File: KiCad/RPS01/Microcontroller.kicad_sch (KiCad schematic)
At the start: 24 parts, among them J1 ISCP, J2 Serial, J22 RGB LED, J3 i2c, J4 Aref, J5 XT30, J6 Temperture, J7 GPIO, SW1 MCU_Button, U1 ATmega328P-A, U2 AMS1117, U3 ADR02AUJZ-REEL7, Y1 16Mhz Crystal

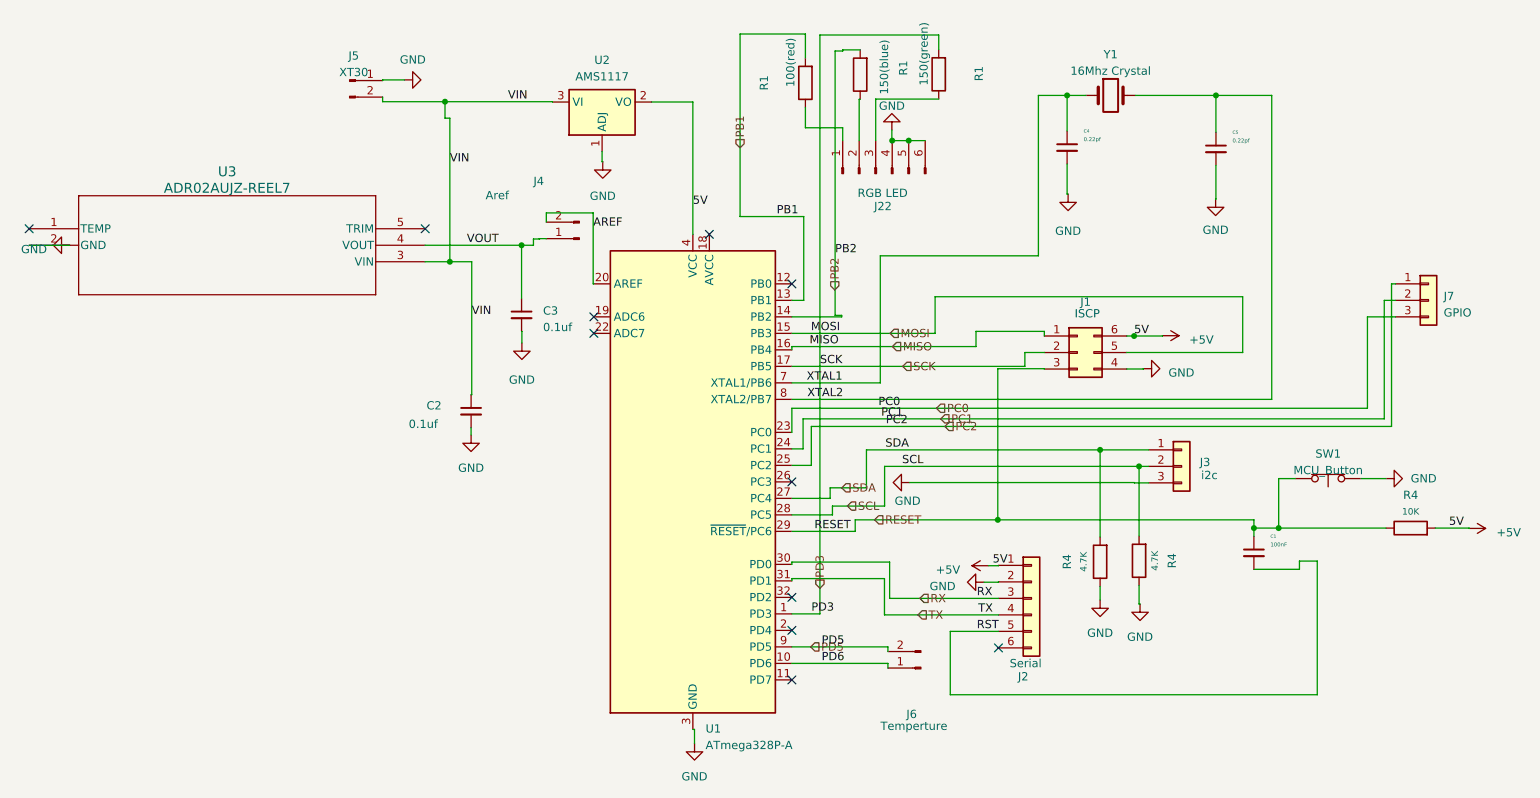
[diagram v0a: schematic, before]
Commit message: Large Schematic Update
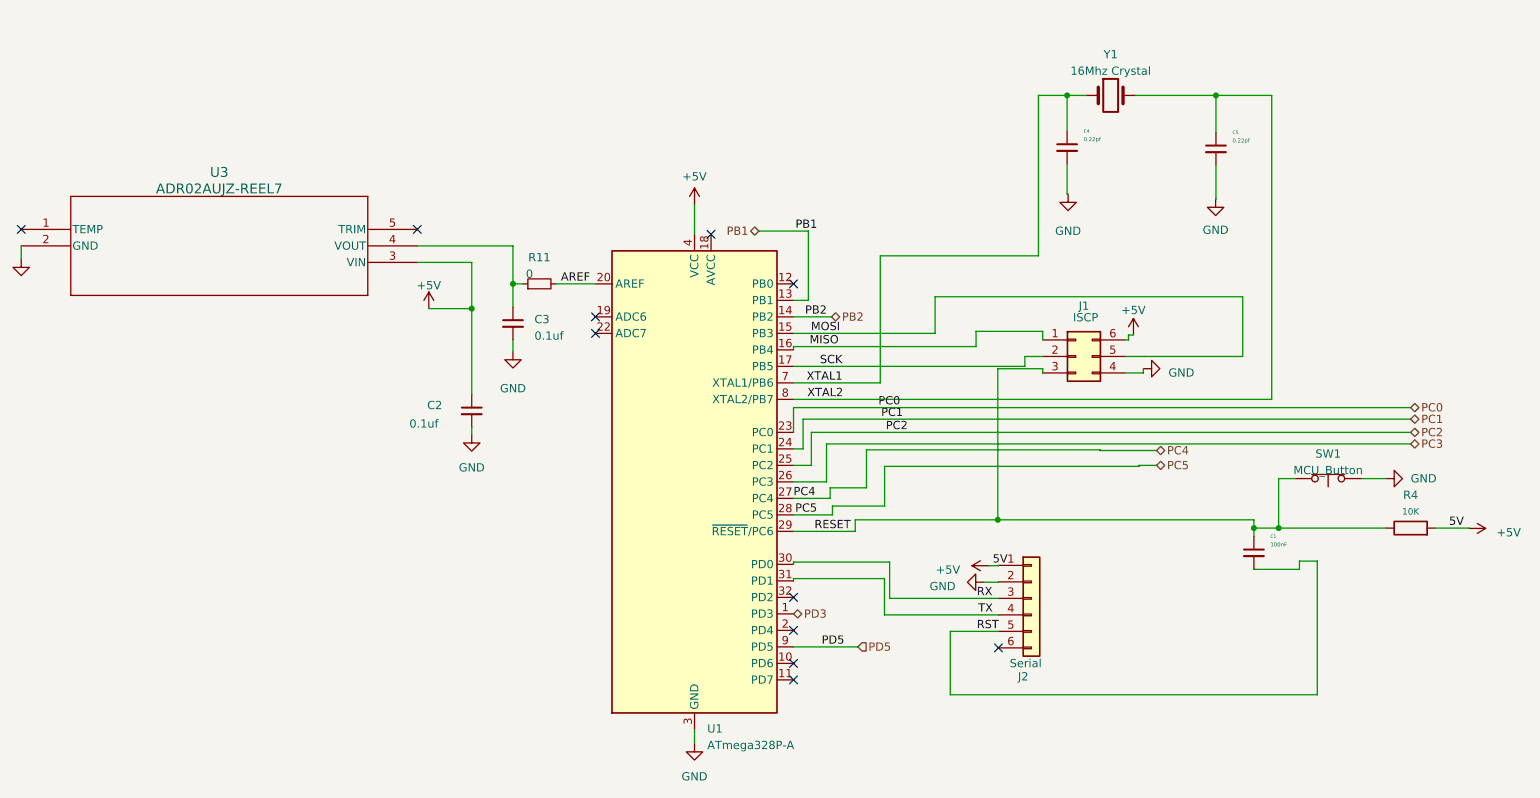
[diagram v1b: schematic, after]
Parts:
- removed J22: RGB LED, LED_SMD:LED_RGB_5050-6, symbol Connector:Conn_01x06_Pin
- removed J3: i2c, Connector_PinHeader_2.54mm:PinHeader_1x02_P2.54mm_Vertical_SMD_Pin1Right, symbol Connector_Generic:Conn_01x03
- removed J4: Aref, Connector_PinHeader_2.54mm:PinHeader_1x02_P2.54mm_Vertical_SMD_Pin1Left, symbol Connector:Conn_01x02_Pin
- removed J5: XT30, Connector_AMASS:AMASS_XT30U-F_1x02_P5.0mm_Vertical, symbol Connector:Conn_01x02_Pin
- removed J6: Temperture, Connector_PinHeader_2.54mm:PinHeader_1x02_P2.54mm_Vertical_SMD_Pin1Left, symbol Connector:Conn_01x02_Pin
- removed J7: GPIO, Connector_PinHeader_2.54mm:PinHeader_1x03_P2.54mm_Vertical_SMD_Pin1Left, symbol Connector_Generic:Conn_01x03
- removed R1: 100(red), Resistor_SMD:R_0603_1608Metric, symbol Device:R
- removed R1: 150(blue), Resistor_SMD:R_0603_1608Metric, symbol Device:R
- removed R1: 150(green), Resistor_SMD:R_0603_1608Metric, symbol Device:R
- removed R4 (x2): 4.7K, Resistor_SMD:R_0603_1608Metric, symbol Device:R
- removed U2: AMS1117, Package_TO_SOT_SMD:SOT-223-3_TabPin2, symbol Regulator_Linear:AMS1117
- added R11: 0, symbol Device:R_Small
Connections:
- net VIN is gone; now on net +5V: C2.1, U3.3 (VIN)
- net AREF: now also R11.2
- net PD3: no longer J1.2 (Pin_2), U1.17 (PB5)
- net PC3: now reaches U1.26 (PC3)
- net PD6: no longer names the net of U1.10 (PD6)
- net SCL renamed PC5
- net SDA renamed PC4
- net VOUT: no longer names the net of C3.1, U3.4 (VOUT)
- net VOUT: now also R11.1
- new net SCK: J1.2 (Pin_2), U1.17 (PB5)
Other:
- moved on the sheet: C3, J1, U3
